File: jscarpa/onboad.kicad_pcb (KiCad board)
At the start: 2 copper layers, 55.6 x 42.3 mm, 11 parts, among them J1 Conn_01x02_Socket, J2 Conn_01x02_Socket, U1 ACS711xLCTR-12AB, U2 mcp6546-e/p

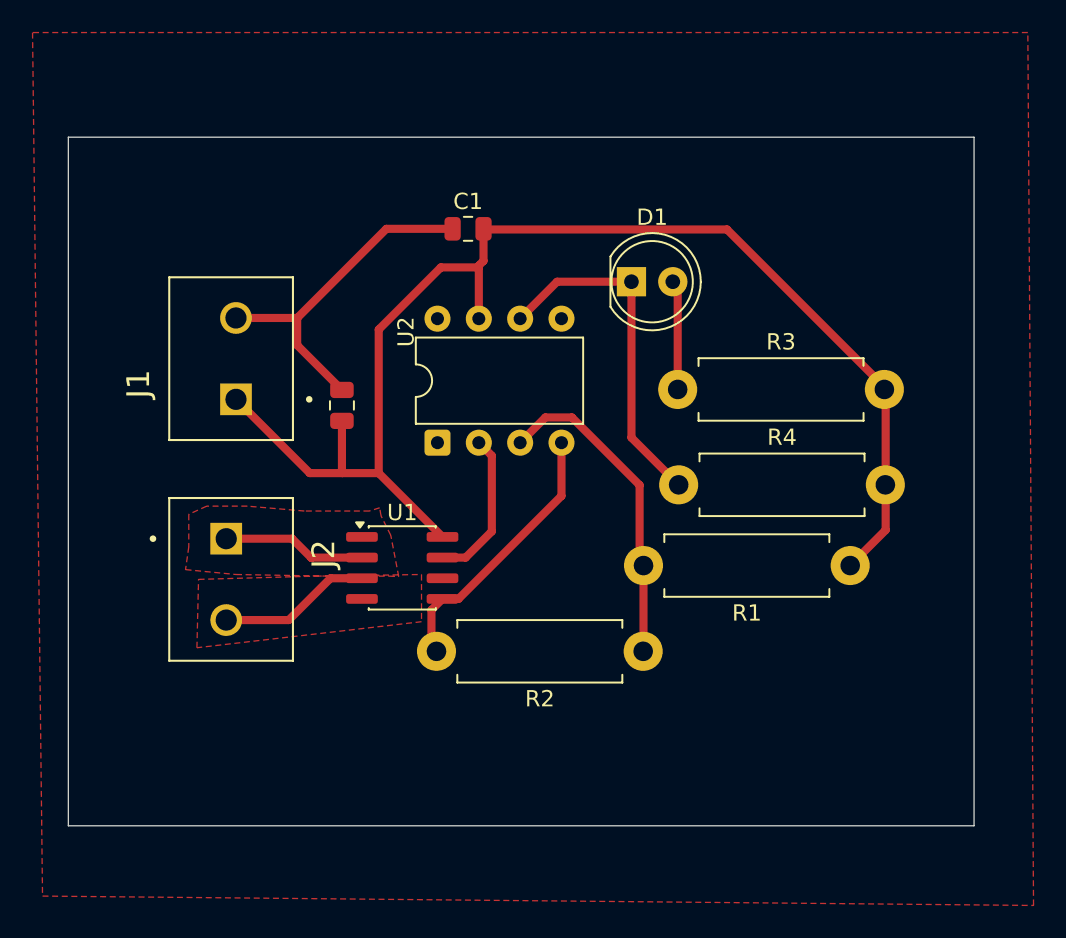
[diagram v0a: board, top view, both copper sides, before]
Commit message: Onboarding: Flipped threw hole components.
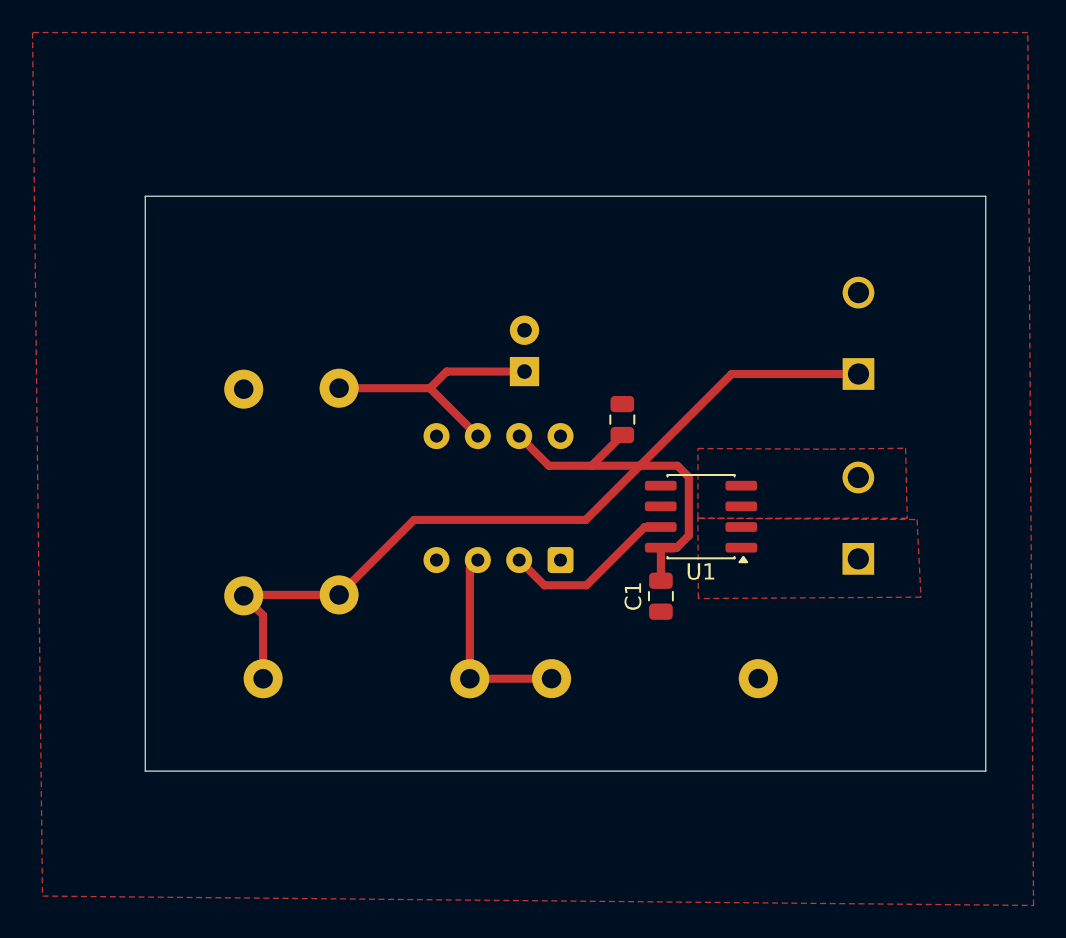
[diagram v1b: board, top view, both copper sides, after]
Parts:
- D1, J1, J2, R1, R2, R3, R4, U2: moved to B.Cu
- moved J2 38.9 mm to (128.7, 95.6), turned to 90 degrees
- moved J1 38.3 mm to (128.8, 84.3)
- moved R1 36.7 mm to (92.2, 103.0), turned to 0 degrees
- moved R3 26.7 mm to (91.0, 85.2), turned to -90 degrees
- moved C1 25.5 mm to (116.6, 97.9), turned to 90 degrees
- moved R4 21.7 mm to (96.8, 85.2), turned to -90 degrees
- moved U1 18.6 mm to (119.1, 93.0), turned to 180 degrees
- moved C2 17.3 mm to (114.2, 87.1)
- moved U2 10.4 mm to (110.4, 95.7)
- moved D1 8.58 mm to (108.2, 84.1), turned to 90 degrees
- moved R2 5.87 mm to (109.9, 103.0), turned to 0 degrees
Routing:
- net GND: track 38.0 -> 0.00 mm
- net +3V3: track 82.2 -> 70.8 mm
- net Current-: track 9.40 -> 0.00 mm
- net Current+: track 8.84 -> 0.00 mm
- net Net-(U2-VIN+): track 20.3 -> 12.5 mm
- net Net-(D1-A): track 6.74 -> 0.00 mm
- net Net-(D1-K): track 21.5 -> 16.0 mm
- net Net-(U1-VIOUT): track 9.48 -> 10.8 mm
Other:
- board size 55.6 x 42.3 mm -> 51.6 x 35.3 mm
